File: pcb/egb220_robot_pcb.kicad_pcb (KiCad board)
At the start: 2 copper layers, 6 parts, among them J1 Conn_01x03_Pin, Q1 Q_Photo_NPN, Q1 SFH309

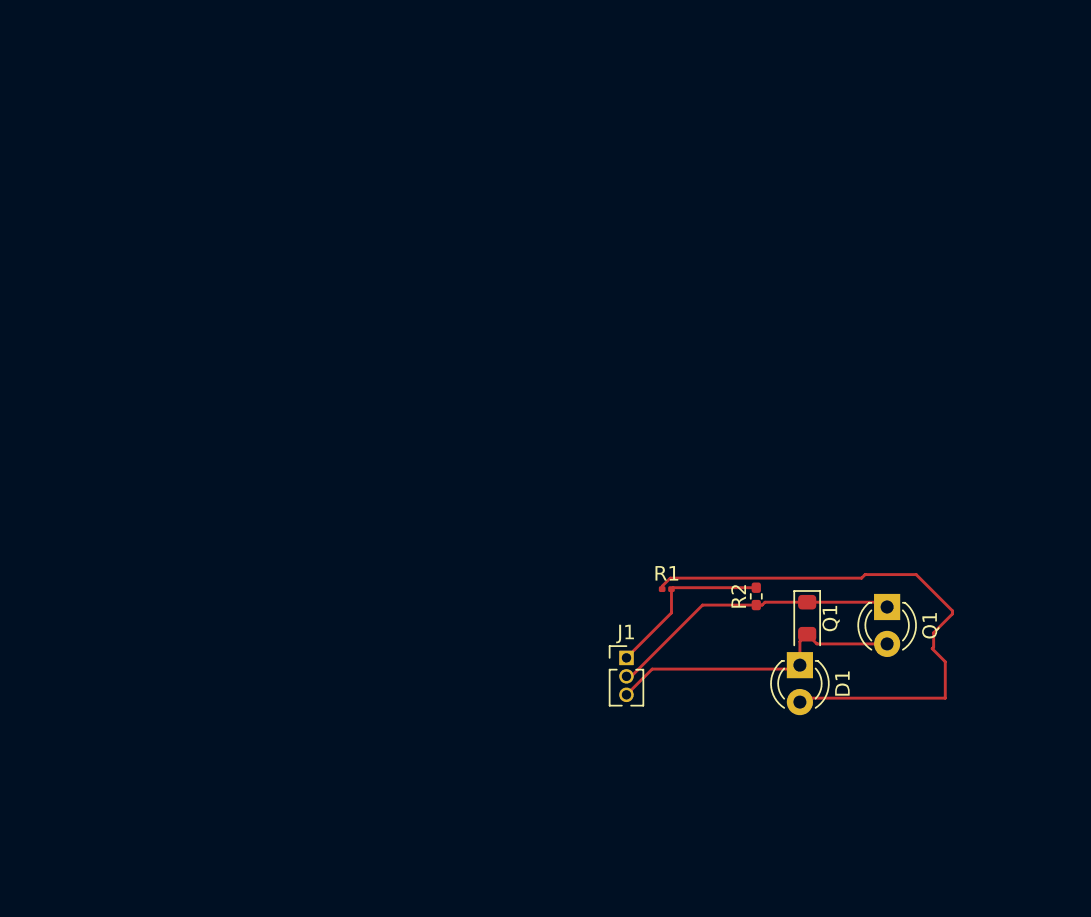
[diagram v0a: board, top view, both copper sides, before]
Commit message: feat(PCB): Completed sensor array and first submission
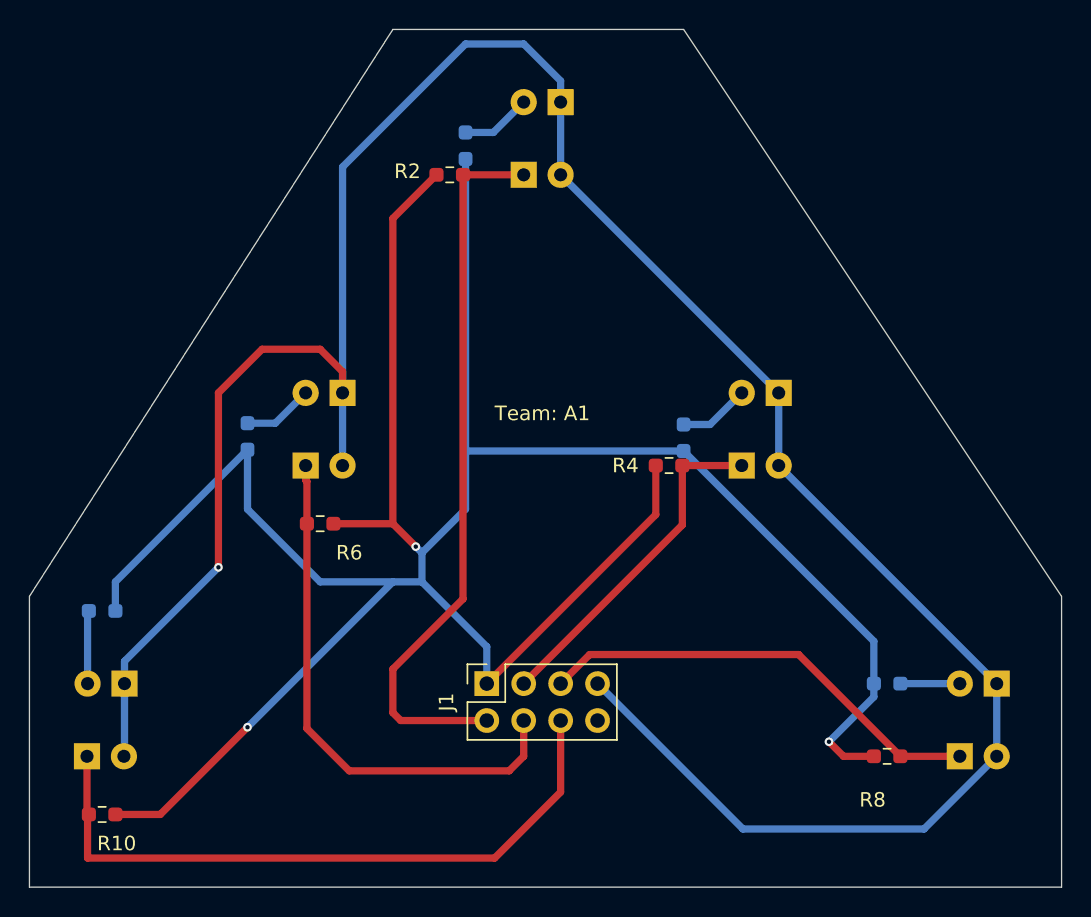
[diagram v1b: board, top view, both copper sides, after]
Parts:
- removed the Q1 at (143.5, 90.5)
- removed the Q1 at (149.0, 89.7)
- added D2: LED, LED_THT:LED_D3.0mm_IRGrey, B.Cu at (141.5, 75.0)
- added D3: LED, LED_THT:LED_D3.0mm_IRGrey, B.Cu at (111.5, 75.0)
- added D4: LED, LED_THT:LED_D3.0mm_IRGrey, B.Cu at (156.5, 95.0)
- added D5: LED, LED_THT:LED_D3.0mm_IRGrey, B.Cu at (96.5, 95.0)
- added Q1: Q_Photo_NPN, LED_THT:LED_D3.0mm_IRBlack, B.Cu at (124.0, 60.0)
- added Q2: Q_Photo_NPN, LED_THT:LED_D3.0mm_IRBlack, B.Cu at (139.0, 80.0)
- added Q3: Q_Photo_NPN, LED_THT:LED_D3.0mm_IRBlack, B.Cu at (109.0, 80.0)
- added Q4: Q_Photo_NPN, LED_THT:LED_D3.0mm_IRBlack, B.Cu at (154.0, 100.0)
- added Q5: Q_Photo_NPN, LED_THT:LED_D3.0mm_IRBlack, B.Cu at (94.0, 100.0)
- added R10: 1M Ohms, Resistor_SMD:R_0603_1608Metric_Pad0.98x0.95mm_HandSolder, F.Cu at (95.0, 104.0)
- added R3: 82 Ohms, Resistor_SMD:R_0603_1608Metric_Pad0.98x0.95mm_HandSolder, B.Cu at (135.0, 78.1)
- added R4: 1M Ohms, Resistor_SMD:R_0603_1608Metric_Pad0.98x0.95mm_HandSolder, F.Cu at (134.0, 80.0)
- added R5: 82 Ohms, Resistor_SMD:R_0603_1608Metric_Pad0.98x0.95mm_HandSolder, B.Cu at (105.0, 78.0)
- added R6: 1M Ohms, Resistor_SMD:R_0603_1608Metric_Pad0.98x0.95mm_HandSolder, F.Cu at (110.0, 84.0)
- added R7: 82 Ohms, Resistor_SMD:R_0603_1608Metric_Pad0.98x0.95mm_HandSolder, B.Cu at (149.0, 95.0)
- added R8: 1M Ohms, Resistor_SMD:R_0603_1608Metric_Pad0.98x0.95mm_HandSolder, F.Cu at (149.0, 100.0)
- added R9: 82 Ohms, Resistor_SMD:R_0603_1608Metric_Pad0.98x0.95mm_HandSolder, B.Cu at (95.0, 90.0)
- D1: footprint LED_THT:LED_D3.0mm -> LED_THT:LED_D3.0mm_IRGrey; moved to B.Cu
- J1: value Conn_01x03_Pin -> Conn_01x07_Socket; footprint Connector_PinHeader_1.27mm:PinHeader_1x03_P1.27mm_Vertical -> Connector_PinSocket_2.54mm:PinSocket_2x04_P2.54mm_Vertical
- R1: value R -> 82 Ohms; footprint Resistor_SMD:R_0201_0603Metric -> Resistor_SMD:R_0603_1608Metric_Pad0.98x0.95mm_HandSolder; moved to B.Cu
- R2: value R -> 1M Ohms; footprint Resistor_SMD:R_0402_1005Metric_Pad0.72x0.64mm_HandSolder -> Resistor_SMD:R_0603_1608Metric_Pad0.98x0.95mm_HandSolder
- moved D1 42.1 mm to (126.5, 55.0), turned to 180 degrees
- moved R2 35.9 mm to (118.9, 60.0), turned to 0 degrees
- moved R1 33.5 mm to (120.0, 58.0), turned to 90 degrees
- moved J1 9.77 mm to (121.5, 95.0), turned to 90 degrees
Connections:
- J1 pad 1: Net-(J1-Pin_1) -> VCC
- J1 pad 2: Net-(J1-Pin_2) -> S1
- J1 pad 3: GND -> S2
- R1 pad 1: Net-(D1-A) -> VCC
- R1 pad 2: Net-(J1-Pin_1) -> Net-(D1-A)
- R2 pad 1: Net-(J1-Pin_2) -> VCC
- R2 pad 2: Net-(J1-Pin_1) -> S1
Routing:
- net VCC: track 0.00 -> 195.1 mm, vias 0 -> 3
- net GND: track 21.0 -> 172.2 mm, vias 0 -> 1
- net S1: track 0.00 -> 49.9 mm
- net S5: track 0.00 -> 46.4 mm
- net S3: track 0.00 -> 37.1 mm
- net Net-(D1-A): track 38.7 -> 4.86 mm
- net S4: track 0.00 -> 31.2 mm
- net S2: track 0.00 -> 23.6 mm
- net Net-(J1-Pin_2): track 20.2 -> 0.00 mm
- net Net-(J1-Pin_1): track 11.9 -> 0.00 mm
- net Net-(D5-A): track 0.00 -> 5.04 mm
- net Net-(D2-A): track 0.00 -> 4.90 mm
- net Net-(D3-A): track 0.00 -> 4.86 mm
- net Net-(D4-A): track 0.00 -> 4.09 mm
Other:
- board outline added: 71 x 59 mm
- board text added: "Team: A1"
- board text removed: "Lachlan Ikeguchi"
